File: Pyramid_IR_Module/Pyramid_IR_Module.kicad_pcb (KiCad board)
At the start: 2 copper layers, 20.3 x 9.5 mm, 8 parts, among them P1 CONN_4, Q1 NPN

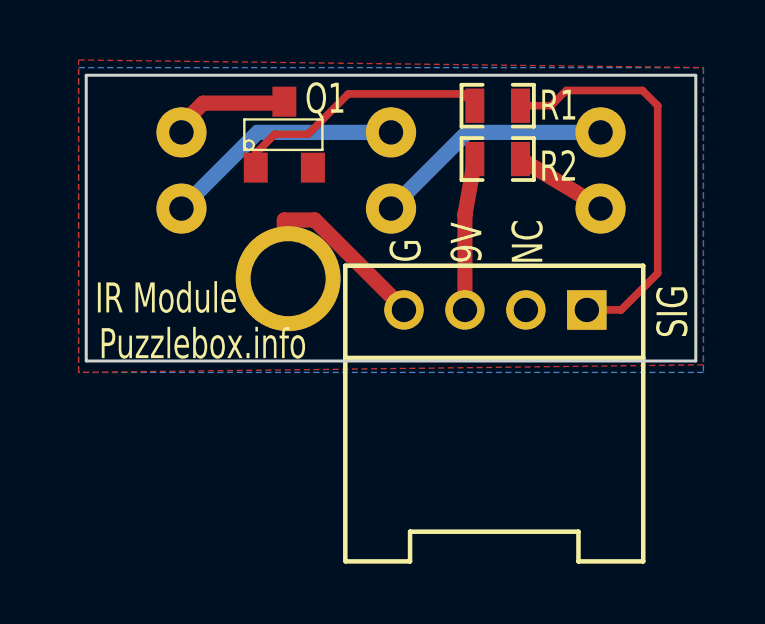
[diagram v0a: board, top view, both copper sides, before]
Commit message: New Product Importing
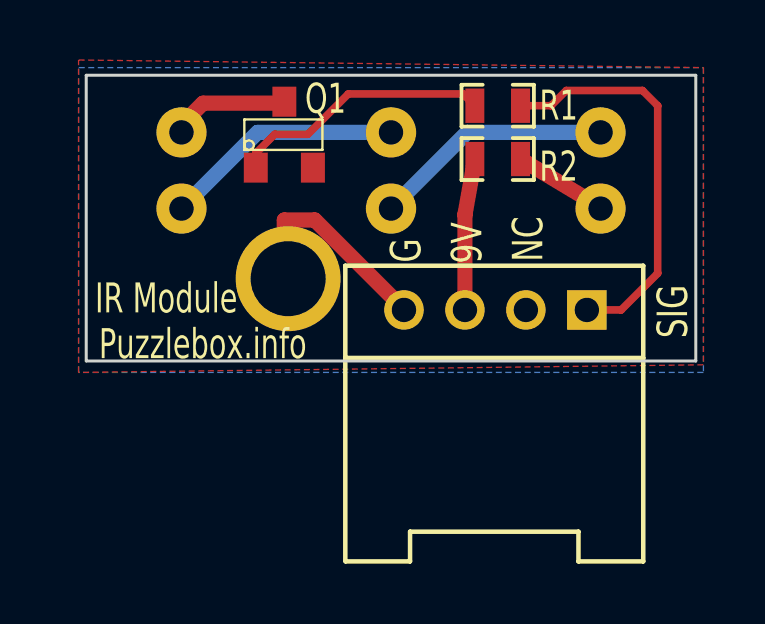
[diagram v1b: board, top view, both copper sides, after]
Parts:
- R1: value 820 -> 820R
- R2: value 82 -> 82R
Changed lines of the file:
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@@
       (effects (font (size 1 0.7) (thickness 0.15)))
     )
-    (fp_text value 82 (at 3.556 0.254) (layer F.SilkS) hide
+    (fp_text value 82R (at 3.556 0.254) (layer F.SilkS) hide
       (effects (font (size 1 0.7) (thickness 0.15)))
     )
@@
       (effects (font (size 1 0.7) (thickness 0.15)))
     )
-    (fp_text value 820 (at -3.81 0 180) (layer F.SilkS) hide
+    (fp_text value 820R (at -3.81 0 180) (layer F.SilkS) hide
       (effects (font (size 1 0.7) (thickness 0.15)))
     )
@@
       (effects (font (size 1.016 0.762) (thickness 0.1524)))
     )
-    (fp_text user NC (at 0.7874 6.096 90) (layer F.SilkS)
+    (fp_text user NC (at 0.889 6.096 90) (layer F.SilkS)
       (effects (font (size 1.016 0.762) (thickness 0.1524)))
     )
